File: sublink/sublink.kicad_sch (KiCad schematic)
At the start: 27 parts

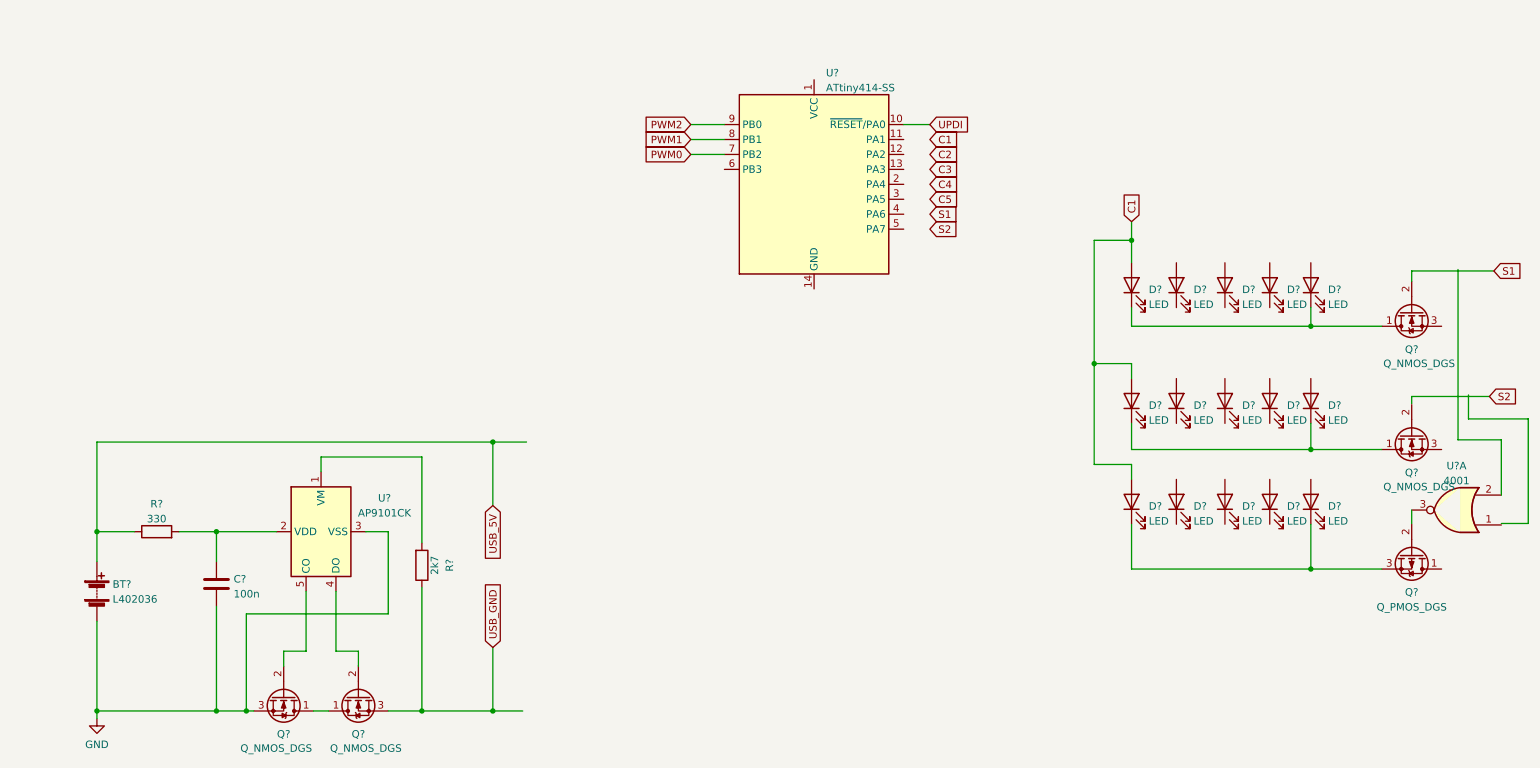
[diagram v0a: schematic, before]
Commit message: wip schematic probably done
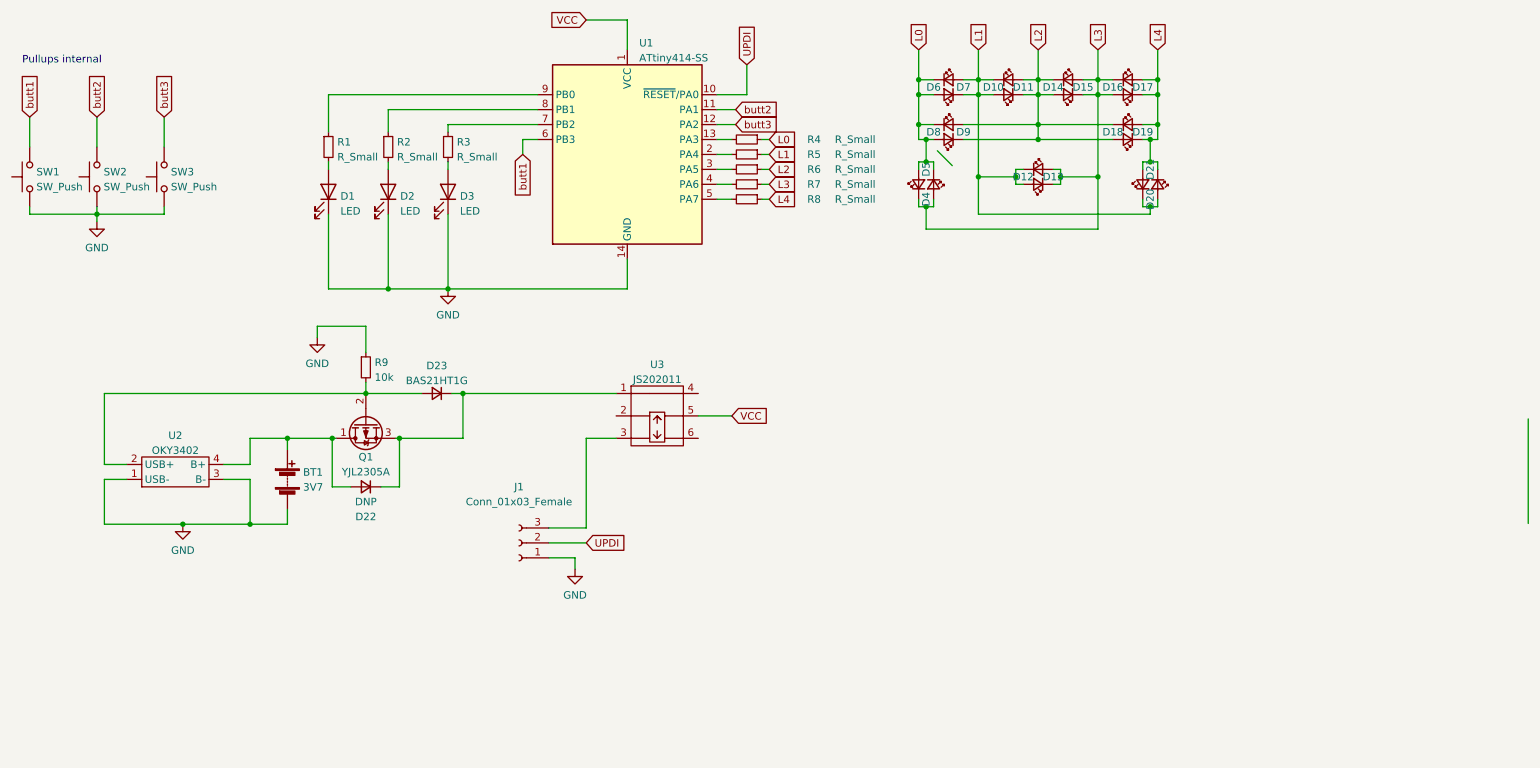
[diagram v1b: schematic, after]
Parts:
- removed BT?: L402036, symbol Device:Battery
- removed C?: 100n, symbol Device:C
- removed D? (x15): LED, symbol Device:LED
- removed Q? (x4): Q_NMOS_DGS, symbol Device:Q_NMOS_DGS
- removed Q?: Q_PMOS_DGS, symbol Device:Q_PMOS_DGS
- removed R?: 330, symbol Device:R
- removed R?: 2k7, symbol Device:R
- removed U?: ATtiny414-SS, Package_SO:SOIC-14_3.9x8.7mm_P1.27mm, symbol MCU_Microchip_ATtiny:ATtiny414-SS
- removed U?: 4001, symbol 4xxx:4001
- removed U?: AP9101CK, Package_TO_SOT_SMD:SOT-23-5, symbol Battery_Management:AP9101CK
- added BT1: 3V7, Connector_PinHeader_2.54mm:PinHeader_1x02_P2.54mm_Vertical, symbol Device:Battery
- added D1, D2, D3: LED, LED_SMD:LED_0805_2012Metric_Pad1.15x1.40mm_HandSolder, symbol Device:LED
- added D10, D11, D12, D13, D14, D15, D16, D17, D18, D19, D20, D21, D4, D5, D6, D7, D8, D9: LED_Small, LED_SMD:LED_0805_2012Metric_Pad1.15x1.40mm_HandSolder, symbol Device:LED_Small
- added D22: DNP, Diode_SMD:D_SOD-323_HandSoldering, symbol Device:D_Small
- added D23: BAS21HT1G, Diode_SMD:D_SOD-323_HandSoldering, symbol Device:D_Small
- added J1: Conn_01x03_Female, Connector_PinHeader_2.54mm:PinHeader_1x03_P2.54mm_Horizontal, symbol Connector:Conn_01x03_Female
- added Q1: YJL2305A, Package_TO_SOT_SMD:SOT-23, symbol Device:Q_PMOS_DGS
- added R1, R2, R3, R4, R5, R6, R7, R8: R_Small, Resistor_SMD:R_0805_2012Metric_Pad1.20x1.40mm_HandSolder, symbol Device:R_Small
- added R9: 10k, Resistor_SMD:R_0805_2012Metric_Pad1.20x1.40mm_HandSolder, symbol Device:R_Small
- added SW1, SW2, SW3: SW_Push, Button_Switch_SMD:SW_SPST_Omron_B3FS-100xP, symbol Switch:SW_Push
- added U1: ATtiny414-SS, Package_SO:SOIC-14_3.9x8.7mm_P1.27mm, symbol MCU_Microchip_ATtiny:ATtiny414-SS
- added U2: OKY3402, sublink_custom:OKY3402, symbol custom_sublink:OKY3402
- added U3: JS202011, sublink_custom:JS202011, symbol custom_sublink:JS202011
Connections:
- net GND: now also BT1.2 (-), D1.1 (K), D2.1 (K), D3.1 (K), J1.1 (Pin_1), R9.1, SW1.1, SW2.1, SW3.1, U1.14 (GND), U2.1 (USB-), U2.3 (B-)
- net UPDI: now also J1.2 (Pin_2), U1.10 (~{RESET}/PA0)
- new net: D23.2 (A), Q1.2 (G), R9.2, U2.2 (USB+)
- new net: BT1.1 (+), D22.2 (A), Q1.1 (D), U2.4 (B+)
- new net: R4.2, U1.13 (PA3)
- new net: J1.3 (Pin_3), U3.3
- new net: D2.2 (A), R2.2
- new net: R6.2, U1.3 (PA5)
- new net: R2.1, U1.8 (PB1)
- new net: R1.1, U1.9 (PB0)
- new net: D1.2 (A), R1.2
- new net: R7.2, U1.4 (PA6)
- new net: D3.2 (A), R3.2
- new net: D22.1 (K), D23.1 (K), Q1.3 (S), U3.1
- new net: R3.1, U1.7 (PB2)
- new net: R5.2, U1.2 (PA4)
- new net: R8.2, U1.5 (PA7)
- new net L0: D4.2 (A), D5.1 (K), D6.1 (K), D7.2 (A), D8.1 (K), D9.2 (A), R4.1
- new net L1: D10.1 (K), D11.2 (A), D12.1 (K), D13.2 (A), D20.1 (K), D21.2 (A), D6.2 (A), D7.1 (K), R5.1
- new net L2: D10.2 (A), D11.1 (K), D14.1 (K), D15.2 (A), D18.1 (K), D19.2 (A), D8.2 (A), D9.1 (K), R6.1
- new net L3: D12.2 (A), D13.1 (K), D14.2 (A), D15.1 (K), D16.1 (K), D17.2 (A), D4.1 (K), D5.2 (A), R7.1
- new net L4: D16.2 (A), D17.1 (K), D18.2 (A), D19.1 (K), D20.2 (A), D21.1 (K), R8.1
- new net VCC: U1.1 (VCC), U3.5
- new net butt1: SW1.2, U1.6 (PB3)
- new net butt2: SW2.2, U1.11 (PA1)
- new net butt3: SW3.2, U1.12 (PA2)
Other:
- note added: "Pullups internal"
